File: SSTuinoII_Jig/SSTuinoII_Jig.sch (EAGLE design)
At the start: 13 parts, among them J1 MuseLab CMSIS-DAP, Q1 BS170

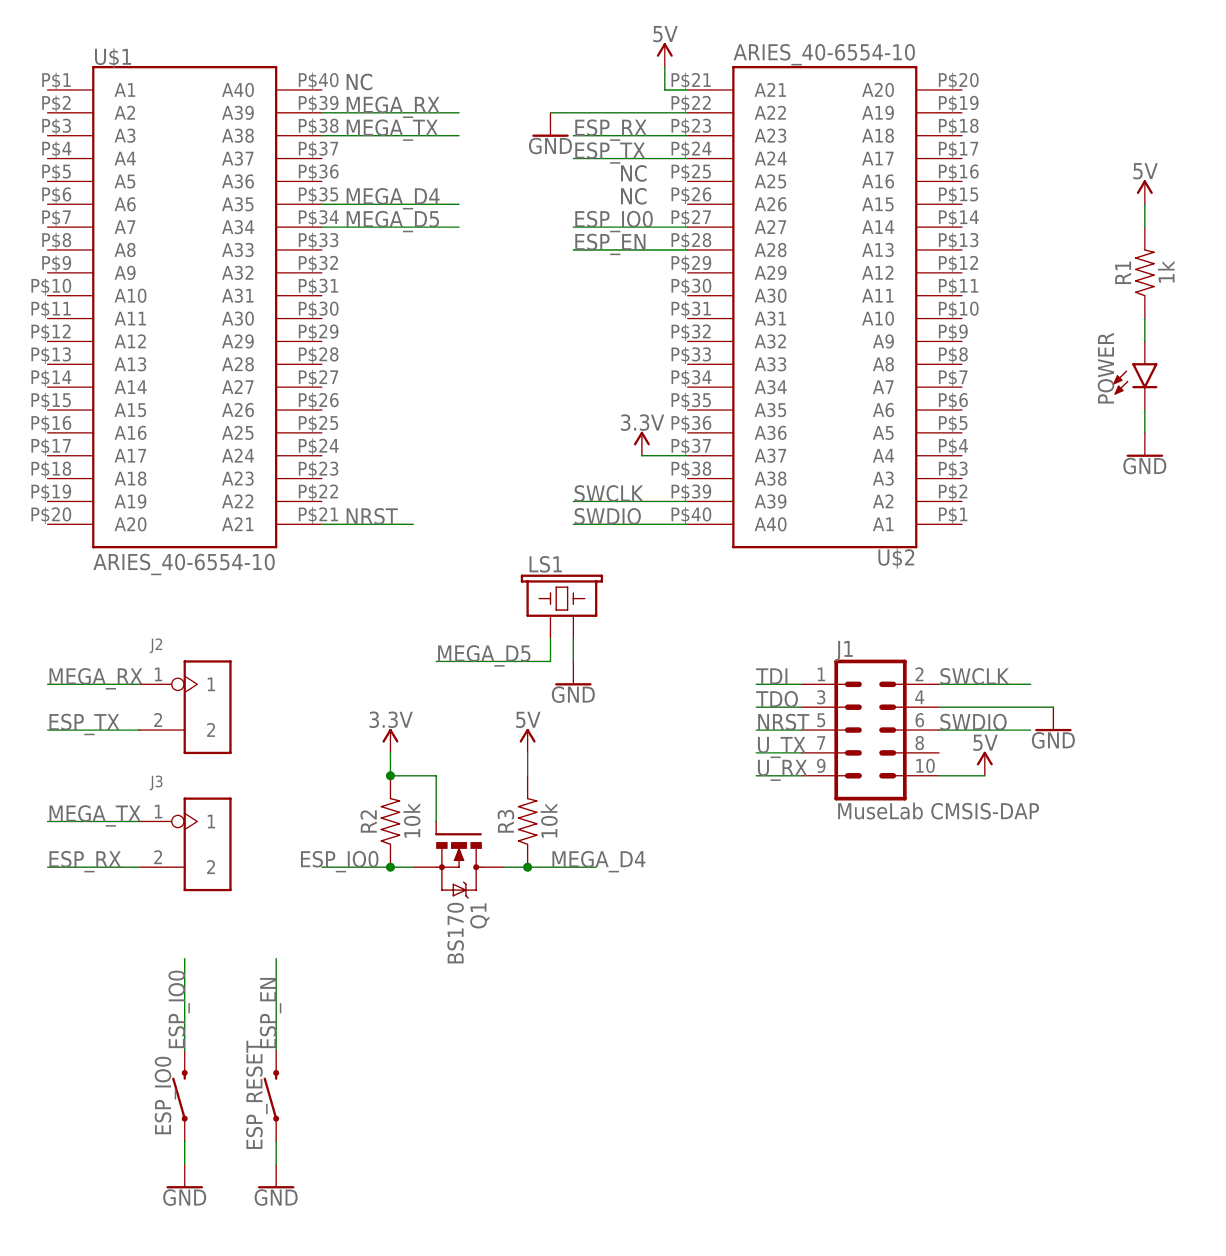
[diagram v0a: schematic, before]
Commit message: finalised test jig
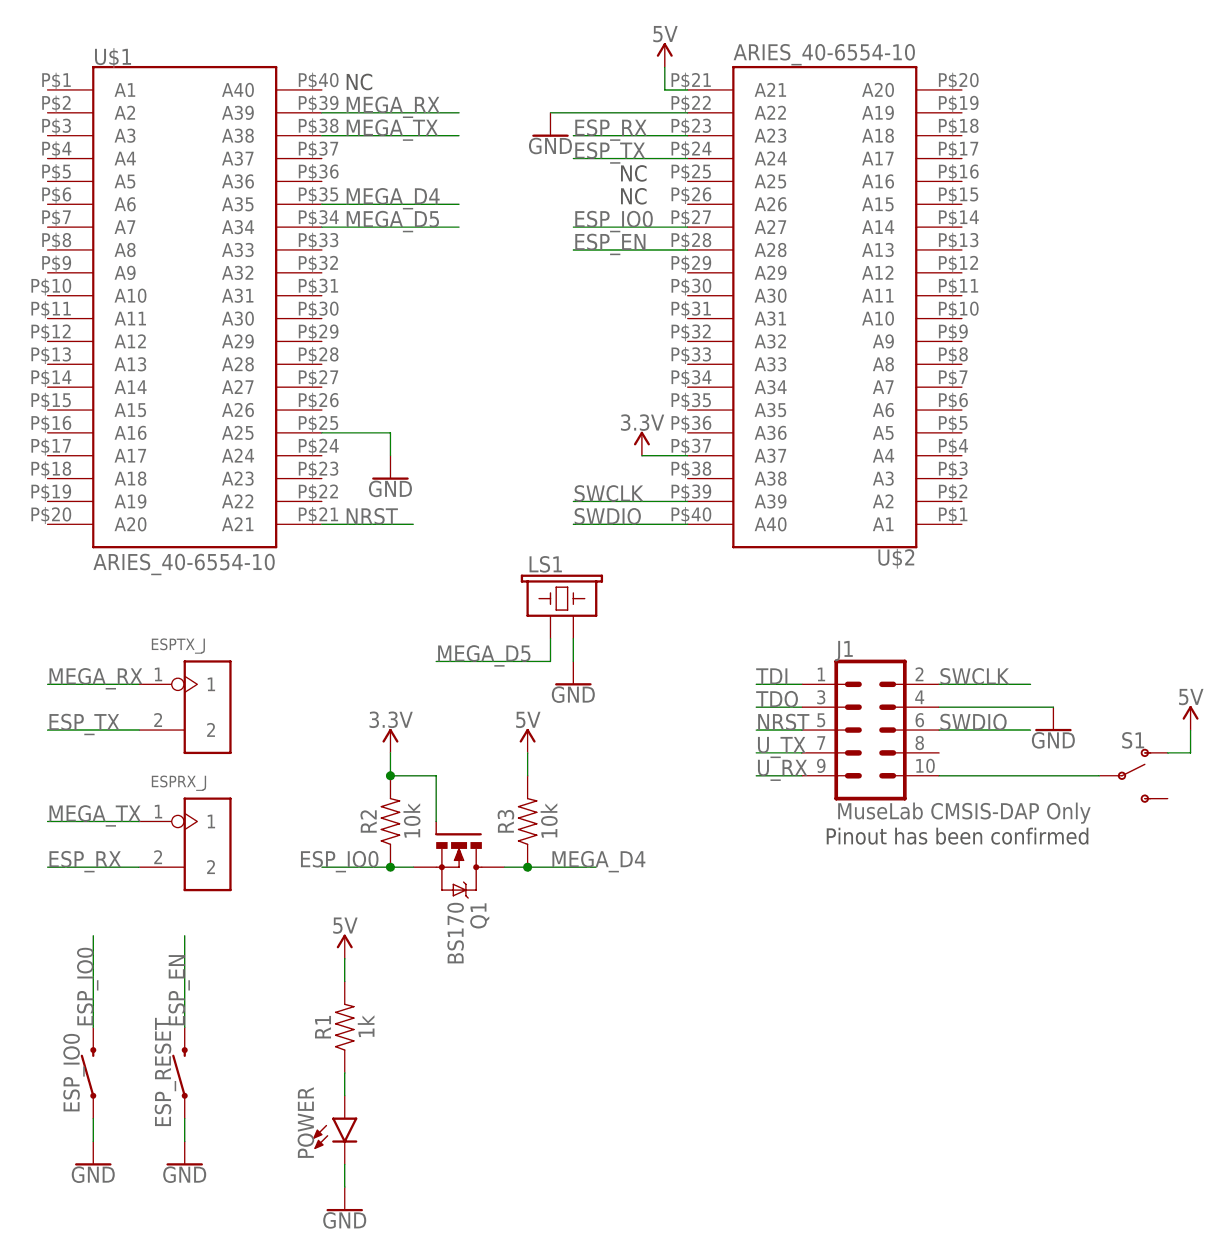
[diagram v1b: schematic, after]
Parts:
- added S1: (no value), SparkFun-Switches:SWITCH-SPDT-PTH-11.6X4.0MM-KIT
- J1: value MuseLab CMSIS-DAP -> MuseLab CMSIS-DAP Only
- renumbered J2 to ESPTX_J, J3 to ESPRX_J
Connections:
- new net PWR: J1.10, S1.P
- net 5V: now also S1.O; no longer J1.10
- net GND: now also U$1.A25
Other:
- note added: "Pinout has been confirmed"
- moved on the sheet: ESP_IO0, ESP_RESET, POWER, R1
